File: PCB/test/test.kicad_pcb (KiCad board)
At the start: 2 copper layers, 44 x 30 mm, 107 parts, among them CN5 UFL, U1 STM32WBxx_QFN48, U2 USBLC6-2SC6, U3 LD3985M33R, X1 NX2016_32MHz, X2 NX2012_32K768Hz

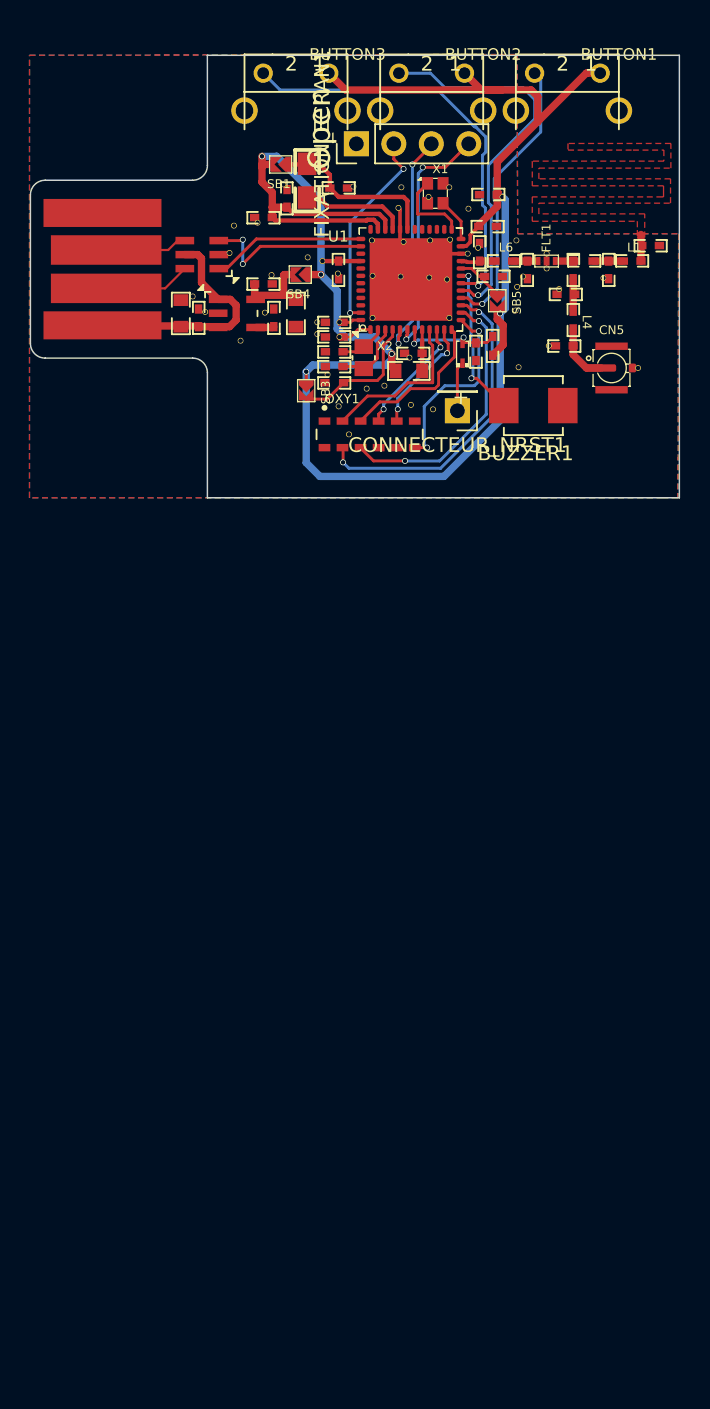
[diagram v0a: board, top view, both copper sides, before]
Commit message: beaucoup de changements
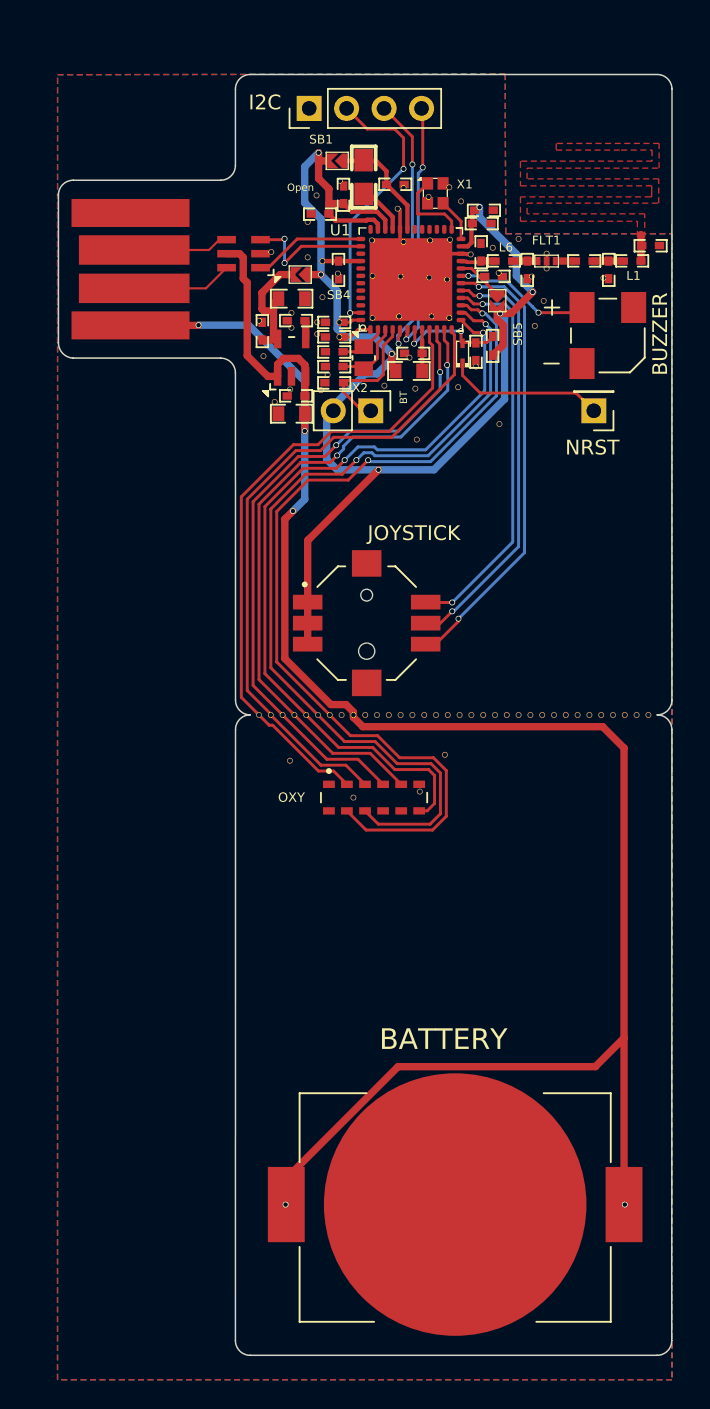
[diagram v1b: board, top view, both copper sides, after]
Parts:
- removed the ? at (144.3, 97.6)
- removed the ? at (142.3, 99.0)
- removed the ? at (135.0, 101.6)
- removed the ? at (136.5, 101.9)
- removed the ? at (142.1, 95.2)
- removed the ? at (139.6, 91.0)
- removed the ? at (130.1, 101.7)
- removed the ? at (134.2, 88.2)
- removed the ? at (138.9, 88.3)
- removed the ? at (123.0, 89.5)
- removed the ? at (141.2, 87.5)
- removed the ? at (145.1, 93.8)
- removed the ? at (142.2, 93.6)
- removed the ? at (150.4, 99.1)
- removed the ? at (132.0, 100.5)
- removed the ? at (123.5, 97.2)
- removed the ? at (134.3, 86.8)
- removed BUTTON1, BUTTON2, BUTTON3: 9-1437565-9, 9-1437565-9:FSMRACD
- removed BUZZER1: CMT-4023S-SMT-TR, CMT-4023S-SMT-TR:CUI_CMT-4023S-SMT-TR
- removed C28, C29, C8: NF, Library:0402_CAP_NPOL
- removed CN5: UFL, Library:UFL
- removed L4: 0R, Library:0402_COIL
- removed SB3: Open, Library:SB-tiny
- added ?: , , F.Cu at (151.1, 122.6)
- added ?: , , F.Cu at (138.4, 87.8)
- added ?: , , F.Cu at (141.5, 122.6)
- added ?: , , F.Cu at (135.3, 100.5)
- added ?: , , F.Cu at (129.0, 94.3)
- added ?: , , F.Cu at (139.1, 122.6)
- added ?: , , F.Cu at (136.7, 122.6)
- added ?: , , F.Cu at (130.3, 122.6)
- added ?: , , F.Cu at (135.6, 127.8)
- added ?: , , F.Cu at (140.7, 122.6)
- added ?: , , F.Cu at (145.5, 122.6)
- added ?: , , F.Cu at (126.8, 125.7)
- added ?: , , F.Cu at (127.1, 122.6)
- added ?: , , F.Cu at (134.1, 88.3)
- added ?: , , F.Cu at (127.9, 122.6)
- added ?: , , F.Cu at (147.1, 122.6)
- added ?: , , F.Cu at (140.9, 92.7)
- added ?: , , F.Cu at (150.3, 122.6)
- added ?: , , F.Cu at (137.3, 125.3)
- added ?: , , F.Cu at (138.2, 100.4)
- added ?: , , F.Cu at (144.7, 122.6)
- added ?: , , F.Cu at (142.3, 122.6)
- added ?: , , F.Cu at (128.0, 89.2)
- added ?: , , F.Cu at (141.0, 102.9)
- added ?: , , F.Cu at (143.1, 122.6)
- added ?: , , F.Cu at (129.5, 122.6)
- added ?: , , F.Cu at (133.5, 122.6)
- added ?: , , F.Cu at (143.9, 122.6)
- added ?: , , F.Cu at (148.7, 122.6)
- added ?: , , F.Cu at (128.9, 100.6)
- added ?: , , F.Cu at (143.4, 96.2)
- added ?: , , F.Cu at (135.4, 104.0)
- added ?: , , F.Cu at (136.4, 95.6)
- added ?: , , F.Cu at (137.5, 122.6)
- added ?: , , F.Cu at (135.9, 122.6)
- added ?: , , F.Cu at (144.0, 94.5)
- added ?: , , F.Cu at (126.9, 95.4)
- added ?: , , F.Cu at (125.0, 98.3)
- added ?: , , F.Cu at (138.3, 122.6)
- added ?: , , F.Cu at (134.2, 95.6)
- added ?: , , F.Cu at (126.3, 122.6)
- added ?: , , F.Cu at (147.9, 122.6)
- added ?: , , F.Cu at (139.4, 99.0)
- added ?: , , F.Cu at (146.3, 122.6)
- added ?: , , F.Cu at (139.9, 122.6)
- added ?: , , F.Cu at (124.7, 122.6)
- added ?: , , F.Cu at (135.1, 122.6)
- added ?: , , F.Cu at (132.7, 122.6)
- added ?: , , F.Cu at (140.6, 91.0)
- added ?: , , F.Cu at (128.7, 122.6)
- added ?: , , F.Cu at (149.5, 122.6)
- added ?: , , F.Cu at (134.3, 122.6)
- added ?: , , F.Cu at (131.1, 122.6)
- added ?: , , F.Cu at (125.5, 122.6)
- added ?: , , F.Cu at (131.9, 122.6)
- added BATTERY: BAT-HLD-002-SMT, BAT-HLD-002-SMT:BAT_BAT-HLD-002-SMT, F.Cu at (138.0, 155.8)
- added BT: Conn_01x02_Male, Connector_PinHeader_2.54mm:PinHeader_1x02_P2.54mm_Vertical, F.Cu at (132.3, 102.0)
- added BUZZER: KSSG13J12-N, KSSG13J12-N:XDCR_KSSG13J12-N, F.Cu at (148.3, 96.9)
- added JOYSTICK: JS1400AFQ, JS1400AFQ:SW_JS1400AFQ, F.Cu at (132.0, 116.4)
- C1, C2: footprint Library:0402_CAP_NPOL -> Passive.PcbLib:0402_CAP_NPOL
- moved ? 24.6 mm to (131.1, 128.2)
- moved OXY 24.6 mm to (132.5, 128.2)
- moved C23 10.1 mm to (126.9, 102.2), turned to 0 degrees
- moved NRST 9.25 mm to (147.4, 102.0)
- moved ? 9.06 mm to (125.8, 101.4), turned to 90 degrees
- moved C24 8.47 mm to (127.2, 101.0), turned to 0 degrees
- moved ? 7.80 mm to (126.8, 100.5), turned to 90 degrees
- moved U3 4.77 mm to (126.9, 98.4), turned to 90 degrees
- moved ? 4.41 mm to (128.6, 87.4)
- moved I2C 4.00 mm to (128.1, 81.5)
- moved L2 3.85 mm to (131.8, 85.0)
- moved ? 3.85 mm to (130.2, 86.4)
- moved C10 3.85 mm to (133.9, 86.7)
- moved C16 3.85 mm to (128.8, 88.7)
- moved C9 3.85 mm to (130.4, 87.4)
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- renumbered FIXATION_ECRAN1 to I2C, CONNECTEUR_NRST1 to NRST, OXY1 to OXY
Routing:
- net 5V_USB: track 16.2 -> 136.2 mm, vias 0 -> 5
- net PA5: track 18.2 -> 58.9 mm
- net PA4: track 13.1 -> 53.0 mm
- net PA6: track 21.7 -> 61.5 mm
- net PA2: track 7.92 -> 44.8 mm
- net PA1: track 8.04 -> 44.0 mm
- net PA3: track 10.6 -> 44.3 mm
- net PA0: track 10.9 -> 43.3 mm
- net 3V3: track 131.7 -> 99.6 mm, vias 5 -> 7
- net PA7: track 19.3 -> 27.1 mm, vias 1 -> 2
- net NRST: track 3.37 -> 10.7 mm
- net Net-(FIXATION_ECRAN1-Pad2): track 14.0 -> 18.8 mm
- net Net-(C29-Pad1): track 4.04 -> 0.00 mm
- net Net-(C10-Pad1): track 11.7 -> 7.72 mm
- net Net-(L2-Pad2): track 7.19 -> 3.45 mm
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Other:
- board size 44 x 30 mm -> 41.6 x 86.8 mm
